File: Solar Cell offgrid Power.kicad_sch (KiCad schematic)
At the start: 3 parts, among them J1 Conn_01x10_Socket, J2 Conn_01x10_Pin, J3 Screw_Terminal_01x02

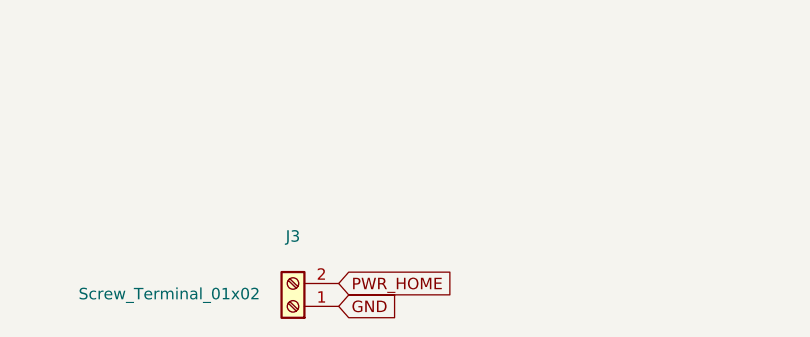
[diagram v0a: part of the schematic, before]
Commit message: Add files via upload
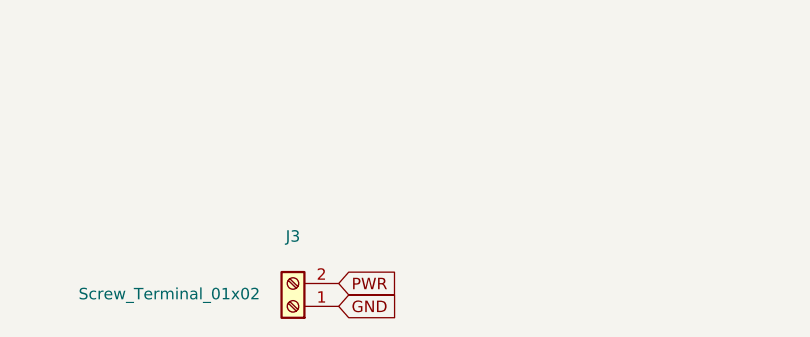
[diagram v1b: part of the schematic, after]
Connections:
- net PWR_HOME is gone; now on net PWR: J3.2 (Pin_2)
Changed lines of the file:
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@@
     )
   )
-  (global_label "PWR_HOME" (shape input) (at 98.3996 106.8324 0) (fields_autoplaced)
+  (global_label "PWR" (shape input) (at 98.3996 106.8324 0) (fields_autoplaced)
     (effects (font (size 1.27 1.27)) (justify left))
-    (property "Intersheetrefs" "${INTERSHEET_REFS}" (at 111.5258 106.8324 0)
+    (property "Intersheetrefs" "${INTERSHEET_REFS}" (at 105.2968 106.8324 0)
       (effects (font (size 1.27 1.27)) (justify left) hide)
     )
